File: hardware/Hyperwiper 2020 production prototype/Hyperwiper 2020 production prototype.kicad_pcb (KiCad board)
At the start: 2 copper layers, 79.5 x 59.1 mm, 17 parts, among them K1 Main Power relay, K2 Wiper control relay, Q1 PN2222A, U1 Teensy4.0, U3 L7805

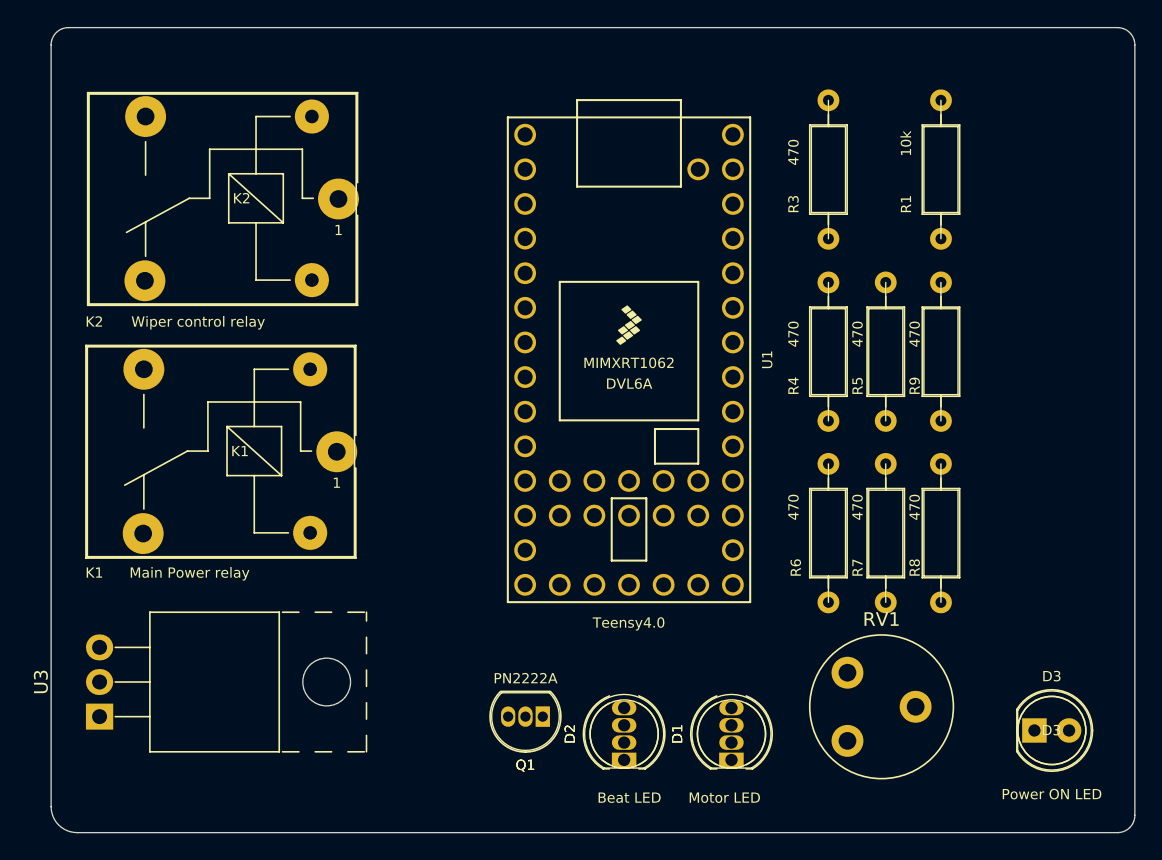
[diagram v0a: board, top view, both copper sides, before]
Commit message: Updated Schematic and board.
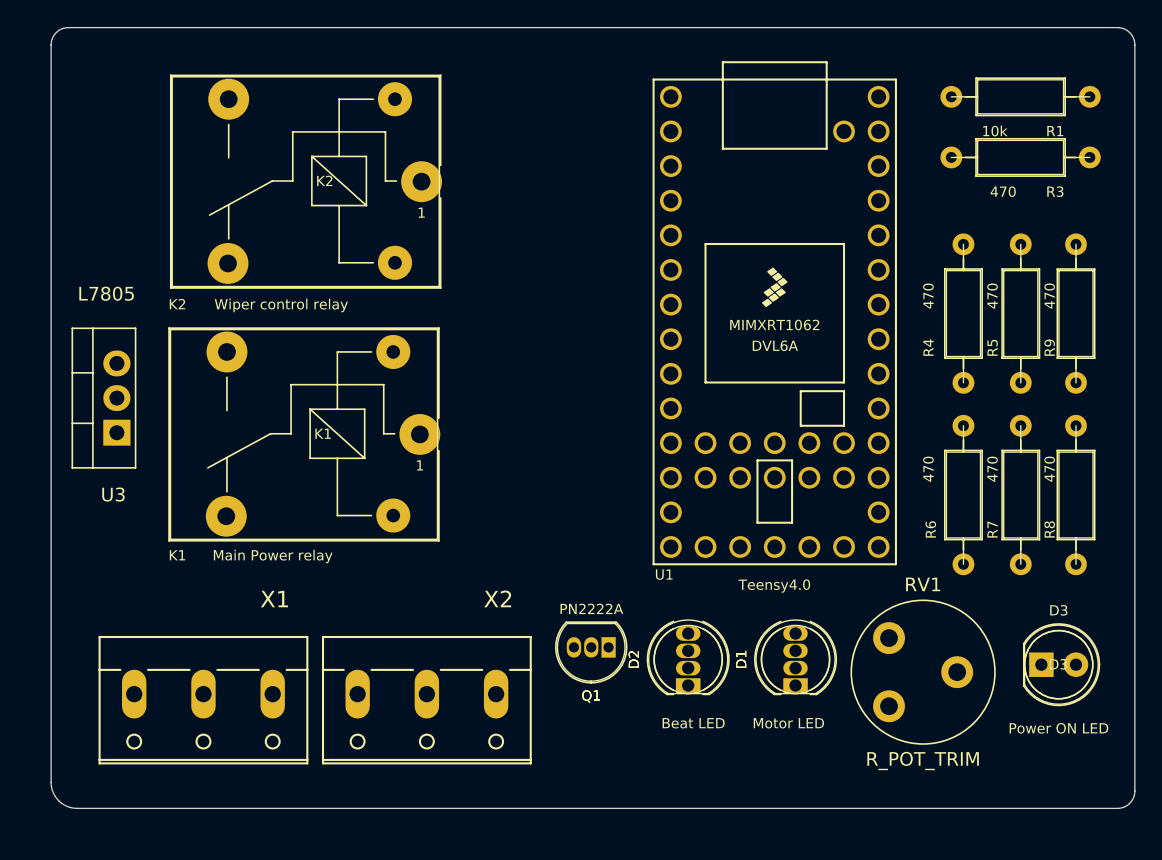
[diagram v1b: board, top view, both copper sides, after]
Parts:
- added X1: W237-3E-bGeigieNanoKit_V1.1r5a-eagle-import, DWP 2020:W237-3E, F.Cu at (910.3, 55.9)
- added X2: W237-3E-bGeigieNanoKit_V1.1r5a-eagle-import, DWP 2020:W237-3E, F.Cu at (926.7, 55.9)
- U3: footprint Package_TO_SOT_THT:TO-220-3_Horizontal_TabUp -> Package_TO_SOT_THT:TO-220-3_Vertical
- moved U3 20.9 mm to (904.0, 36.1)
- moved R3 20.1 mm to (975.4, 15.9), turned to 180 degrees
- moved U1 11.0 mm to (952.2, 27.9)
- moved R4 10.3 mm to (966.1, 32.4)
- moved R6 10.3 mm to (966.1, 45.7)
- moved R8 10.3 mm to (974.3, 45.7)
- moved R9 10.3 mm to (974.3, 32.4)
- moved R5 10.3 mm to (970.3, 32.4)
- moved R7 10.3 mm to (970.3, 45.7)
- moved D1 7.20 mm to (953.8, 54.6)
- moved D2 7.20 mm to (945.9, 54.6)
- moved Q1 7.01 mm to (940.1, 51.8)
- moved K1 6.23 mm to (926.2, 36.2)
- moved K2 6.23 mm to (926.3, 17.7)
- moved D3 4.85 mm to (971.8, 53.1)
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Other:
- board size 79.5 x 59.1 mm -> 79.5 x 57.3 mm
